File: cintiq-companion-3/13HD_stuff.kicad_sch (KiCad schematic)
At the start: 22 parts, among them CN1 13HD_fingerpanel, J2 13HD_buttonboard, X1 13HD_eDP, X2 13HD_penpanel

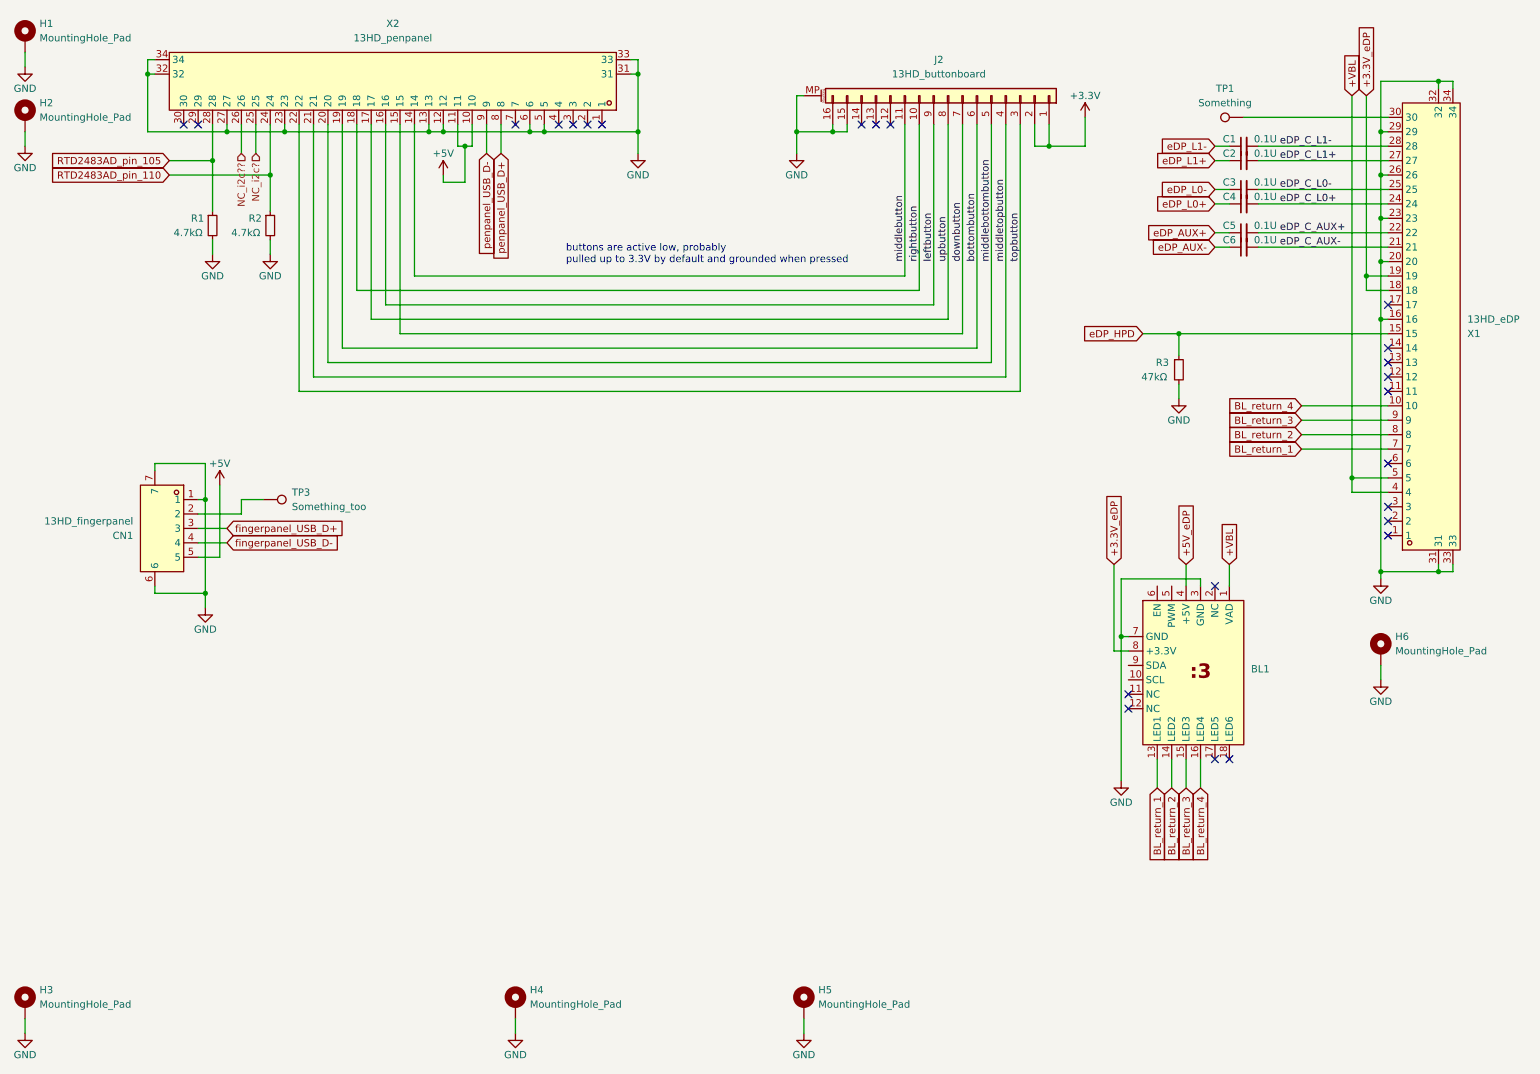
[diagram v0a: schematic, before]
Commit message: susclk
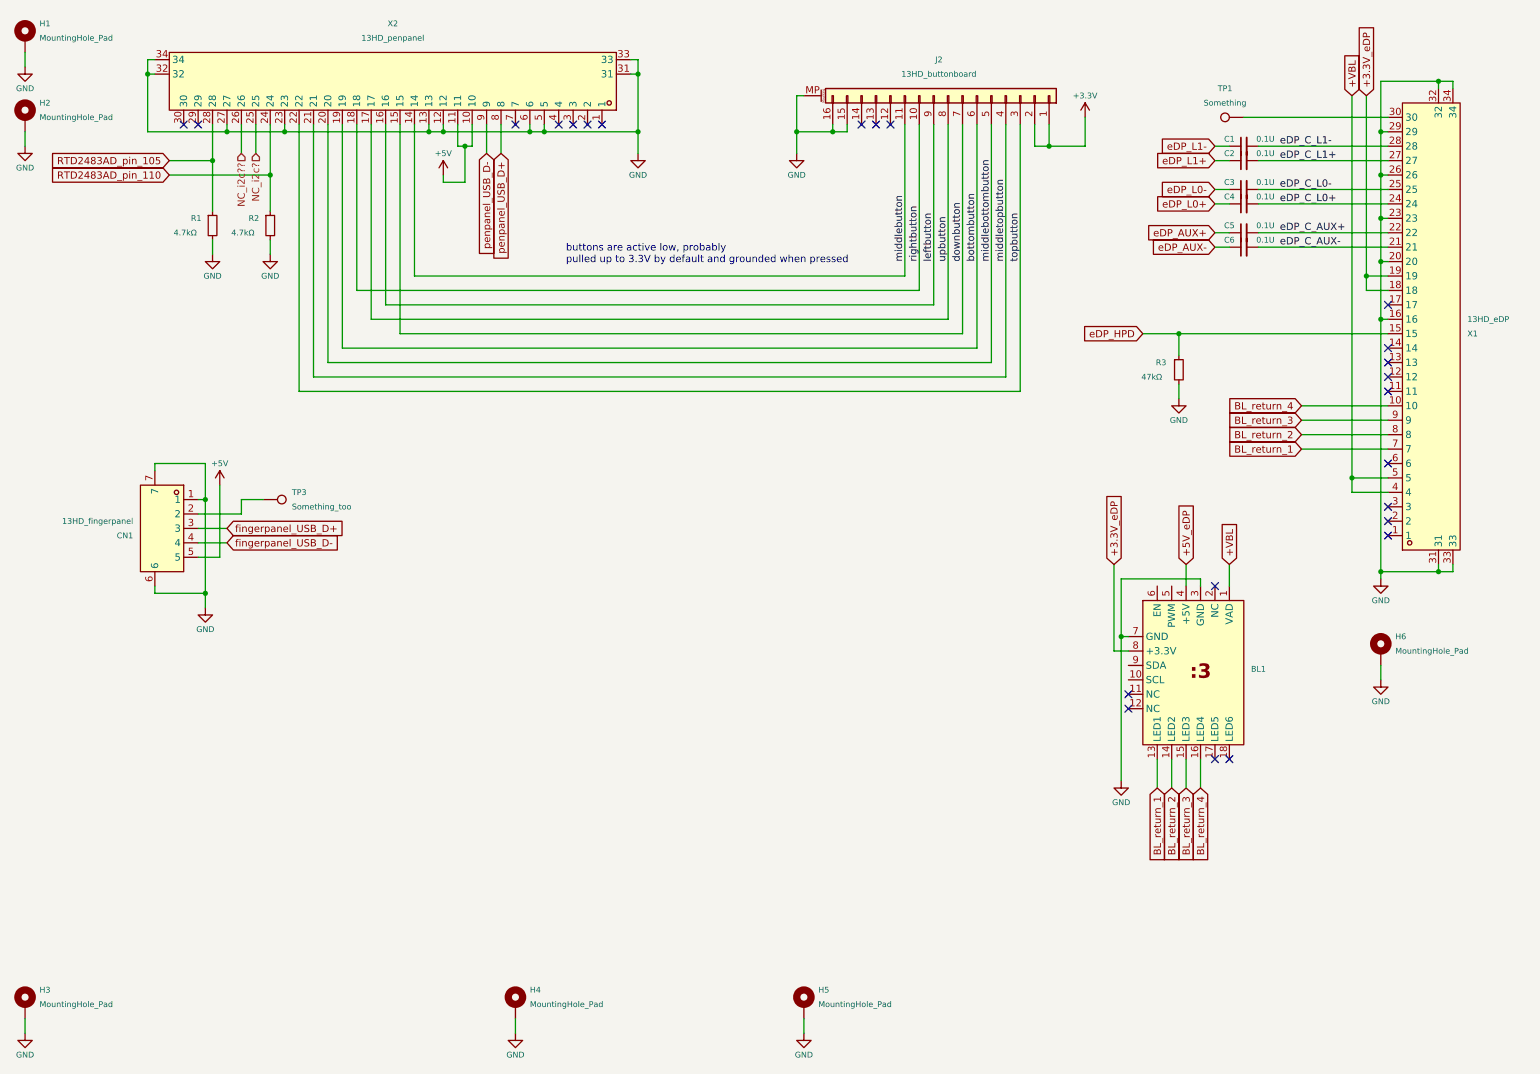
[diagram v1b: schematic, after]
